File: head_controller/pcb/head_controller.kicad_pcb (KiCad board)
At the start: 2 copper layers, 118.1 x 54.6 mm, 64 parts, among them P1 PWR_JACK_2.5x5.5, P2 HEADER_01X03, P3 BNC_DOUBLE_RA, P4 HEADER_02X08_SMD, P5 HEADER_02X08_SMD, P6 HEADER_02X08_SMD, P7 HEADER_02X08_SMD, SW1 SPST_SERIES_M, SW2 KT_SWITCH, U1 MAX6817, U2 MAX6817, U3 TLE723X, U4 TLE723X, U5 TLE723X, U6 TLE723X

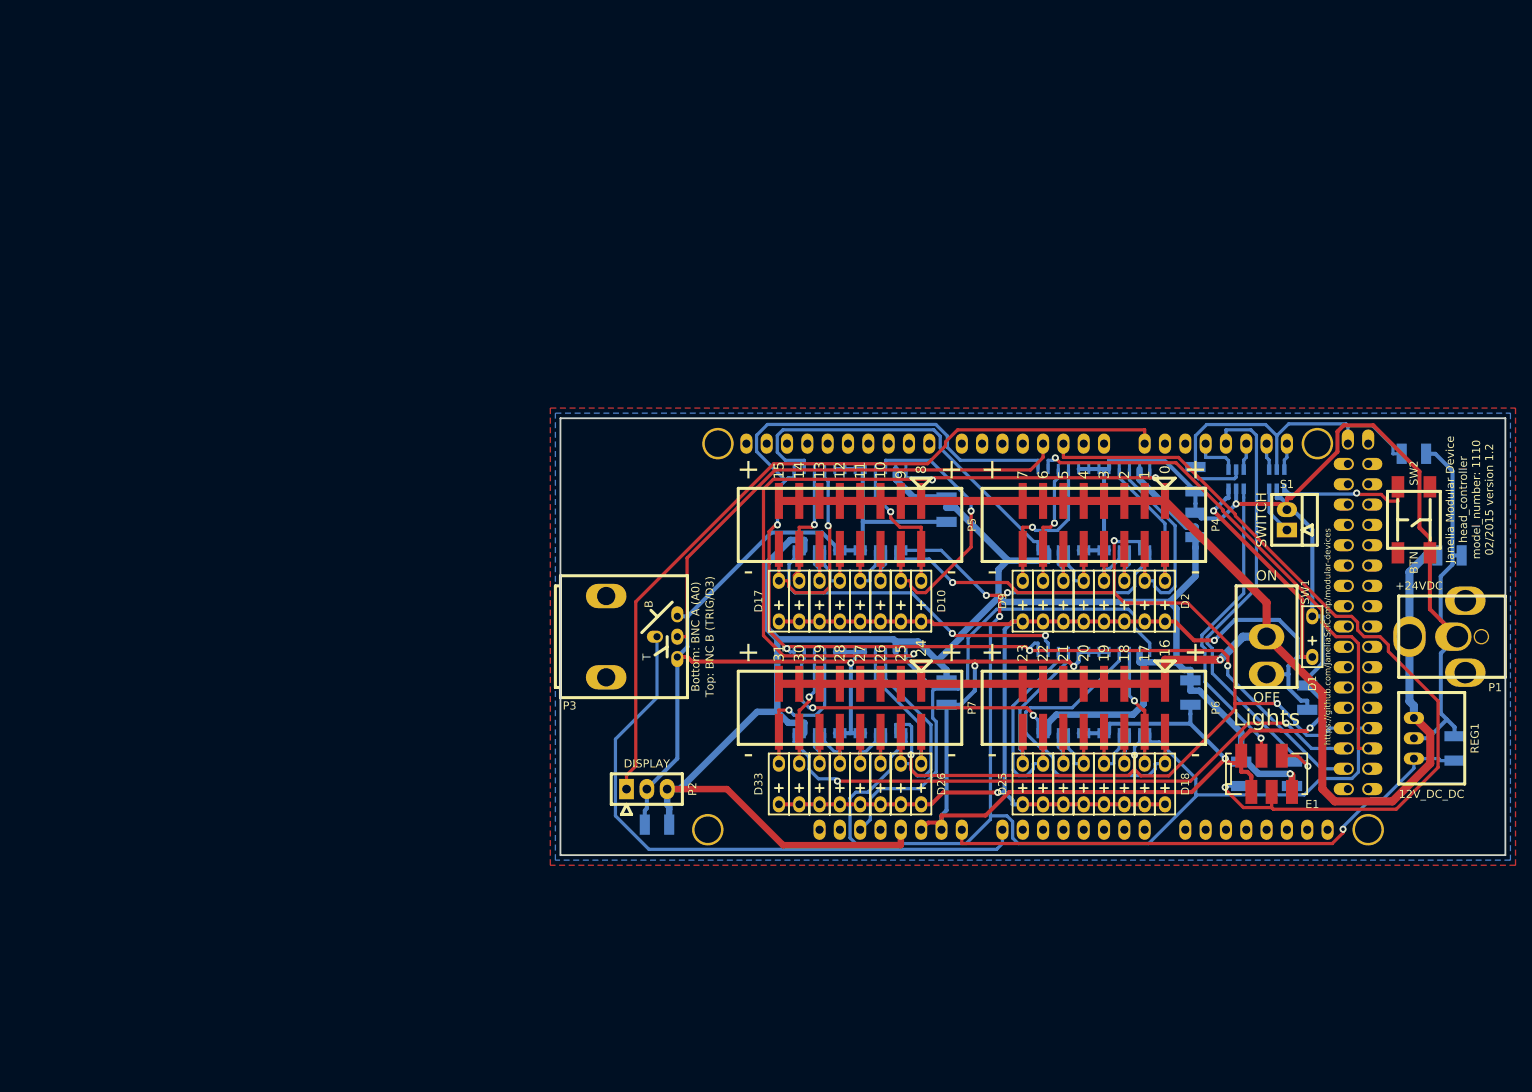
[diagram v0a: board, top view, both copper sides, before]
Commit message: Initial board outline.
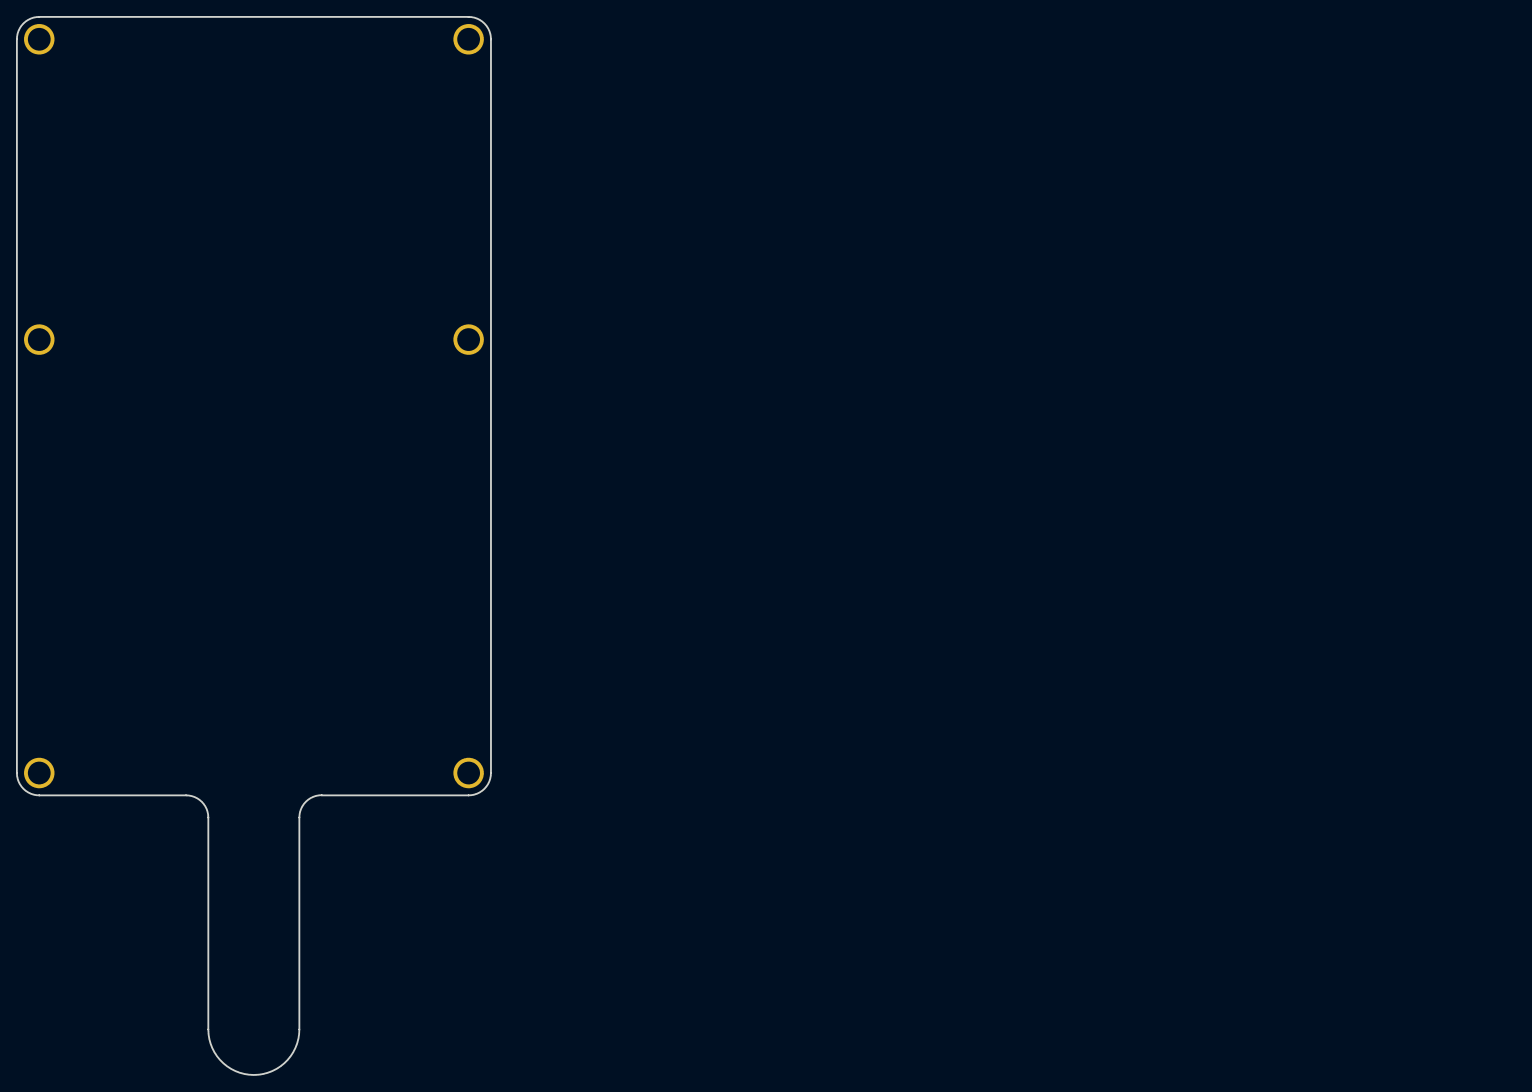
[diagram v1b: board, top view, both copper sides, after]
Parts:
- removed ARDUINO1: ARDUINO_MEGA, head_controller:ARDUINO_MEGA_SHIELD
- removed C1, C2, C3: 10uF, head_controller:SM1210
- removed C4, C5, C6, C7, C8, C9: 0.1uF, head_controller:SM1210
- removed D1, D10, D11, D12, D13, D14, D15, D16, D17, D18, D19, D2, D20, D21, D22, D23, D24, D25, D26, D27, D28, D29, D3, D30, D31, D32, D33, D4, D5, D6, D7, D8, D9: LED_24V, head_controller:LED_555-3XXX
- removed E1: ENCODER_C14, head_controller:Micro-MaTch_6_SMD
- removed P1: PWR_JACK_2.5x5.5, head_controller:DCJACK_2PIN_HIGHCURRENT
- removed P2: HEADER_01X03, footprints:Header_3_Pin
- removed P3: BNC_DOUBLE_RA, head_controller:BNC_DOUBLE
- removed P4, P5, P6, P7: HEADER_02X08_SMD, head_controller:HEADER_02x08_SMD
- removed R1, R2, R3: 5.11k, head_controller:SM1210
- removed REG1: CONV_DC_DC_12V_1A, head_controller:DC_DC_CONV_R78C
- removed S1: HEADER_01X02_SHR, head_controller:Header_Shrouded_2_Pin
- removed SW1: SPST_SERIES_M, head_controller:SPST_SERIES_M
- removed SW2: KT_SWITCH, head_controller:KT_SWITCH
- removed U1, U2: MAX6817, head_controller:MAX6817
- removed U3, U4, U5, U6: TLE723X, head_controller:TLE723X
- added REF**: mounting_hole, head_controller:mounting_hole, F.Cu at (43.2, 55.9)
- added REF**: mounting_hole, head_controller:mounting_hole, F.Cu at (81.3, 27.9)
- added REF**: mounting_hole, head_controller:mounting_hole, F.Cu at (27.9, 66.0)
- added REF**: mounting_hole, head_controller:mounting_hole, F.Cu at (81.3, 66.0)
- added REF**: mounting_hole, head_controller:mounting_hole, F.Cu at (27.9, 119.4)
- added REF**: mounting_hole, head_controller:mounting_hole, F.Cu at (81.3, 119.4)
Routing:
- net GND: track 445.6 -> 0.00 mm, vias 6 -> 0
- net +5V: track 260.3 -> 0.00 mm, vias 1 -> 0
- net VAA: track 203.1 -> 0.00 mm, vias 1 -> 0
- net /LED_PWR: track 184.2 -> 0.00 mm, vias 3 -> 0
- net /CS: track 171.1 -> 0.00 mm, vias 3 -> 0
- net /RST: track 164.0 -> 0.00 mm, vias 3 -> 0
- net /SCK: track 153.6 -> 0.00 mm, vias 4 -> 0
- net /IN: track 141.0 -> 0.00 mm, vias 5 -> 0
- net /ENC_B: track 104.7 -> 0.00 mm, vias 1 -> 0
- net /TX3: track 98.4 -> 0.00 mm
- net /MISO: track 77.6 -> 0.00 mm, vias 2 -> 0
- net /BNC_A: track 76.7 -> 0.00 mm
- net /V_IN: track 69.0 -> 0.00 mm, vias 1 -> 0
- net /MOSI: track 65.0 -> 0.00 mm, vias 1 -> 0
- net /BNC_B: track 62.5 -> 0.00 mm
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- removed copper zone on B.Cu, net GND
- removed copper zone on F.Cu, net VAA
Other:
- board size 118.1 x 54.6 mm -> 59.3 x 132.3 mm
- net class Default: clearance 0.254 -> 0.2; trace_width 0.254 -> 0.25; via_dia 0.889 -> 0.6; via_drill 0.635 -> 0.4
- net class GND removed
- net class LEDPOWER removed
- net class POWER removed
- net class SIGNAL removed
- net class SUPERPOWER removed
- rule pad_to_mask_clearance: 0 -> 0.2
- rule trace_clearance: 0.254 -> 0.2
- rule trace_min: 0.254 -> 0.2
- rule via_min_drill: 0.508 -> 0.3
- rule via_min_size: 0.889 -> 0.4
- board text removed: "+"
- board text removed: "+24VDC"
- board text removed: "-"
- board text removed: "0"
- board text removed: "1"
- board text removed: "10"
- board text removed: "11"
- board text removed: "12"
- board text removed: "12V_DC_DC"
- board text removed: "13"
- board text removed: "14"
- board text removed: "15"
- board text removed: "16"
- board text removed: "17"
- board text removed: "18"
- board text removed: "19"
- board text removed: "2"
- board text removed: "20"
- board text removed: "21"
- board text removed: "22"
- board text removed: "23"
- board text removed: "24"
- board text removed: "25"
- board text removed: "26"
- board text removed: "27"
- board text removed: "28"
- board text removed: "29"
- board text removed: "3"
- board text removed: "30"
- board text removed: "31"
- board text removed: "4"
- board text removed: "5"
- board text removed: "6"
- board text removed: "7"
- board text removed: "8"
- board text removed: "9"
- board text removed: "DISPLAY"
- board text removed: "Janelia Modular Device head_controller model_number: 1110 02/2015 version 1.2"
- board text removed: "SWITCH"
- board text removed: "https://github.com/JaneliaSciComp/modular-devices"
